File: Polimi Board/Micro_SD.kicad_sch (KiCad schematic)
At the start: 6 parts, among them J3 Micro_SD_Card, U4 74LVC125

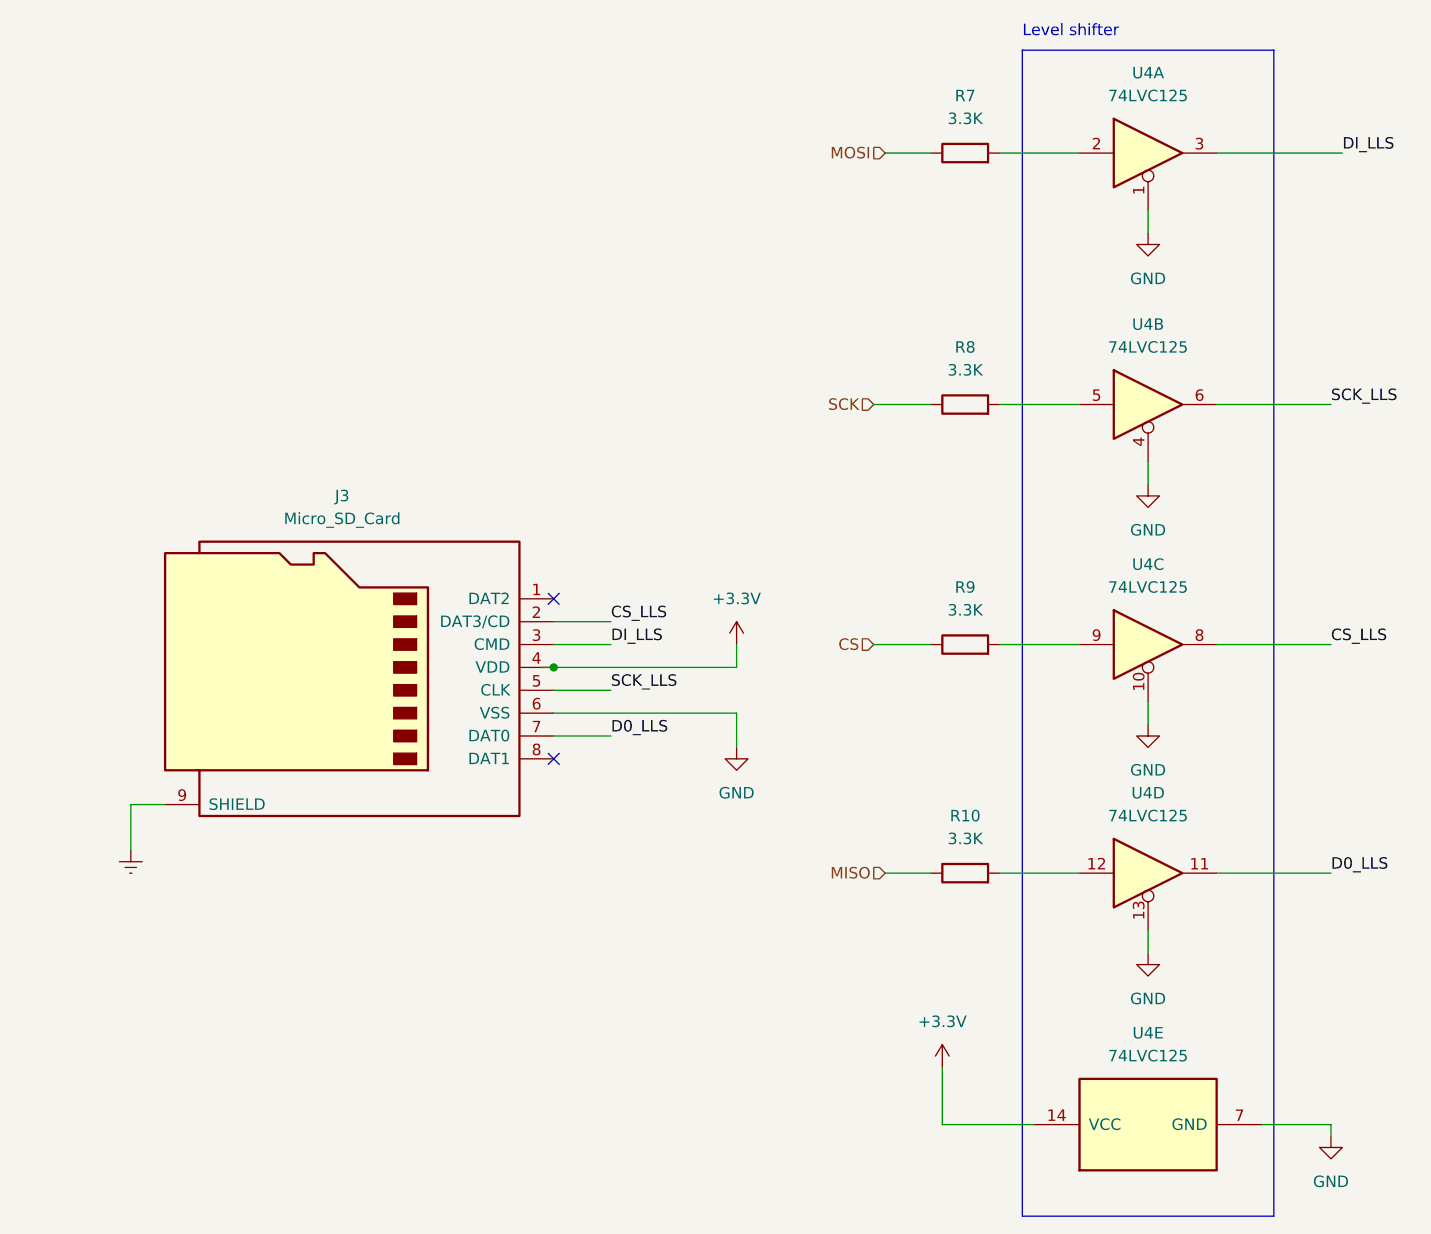
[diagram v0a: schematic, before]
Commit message: Fatte modifiche
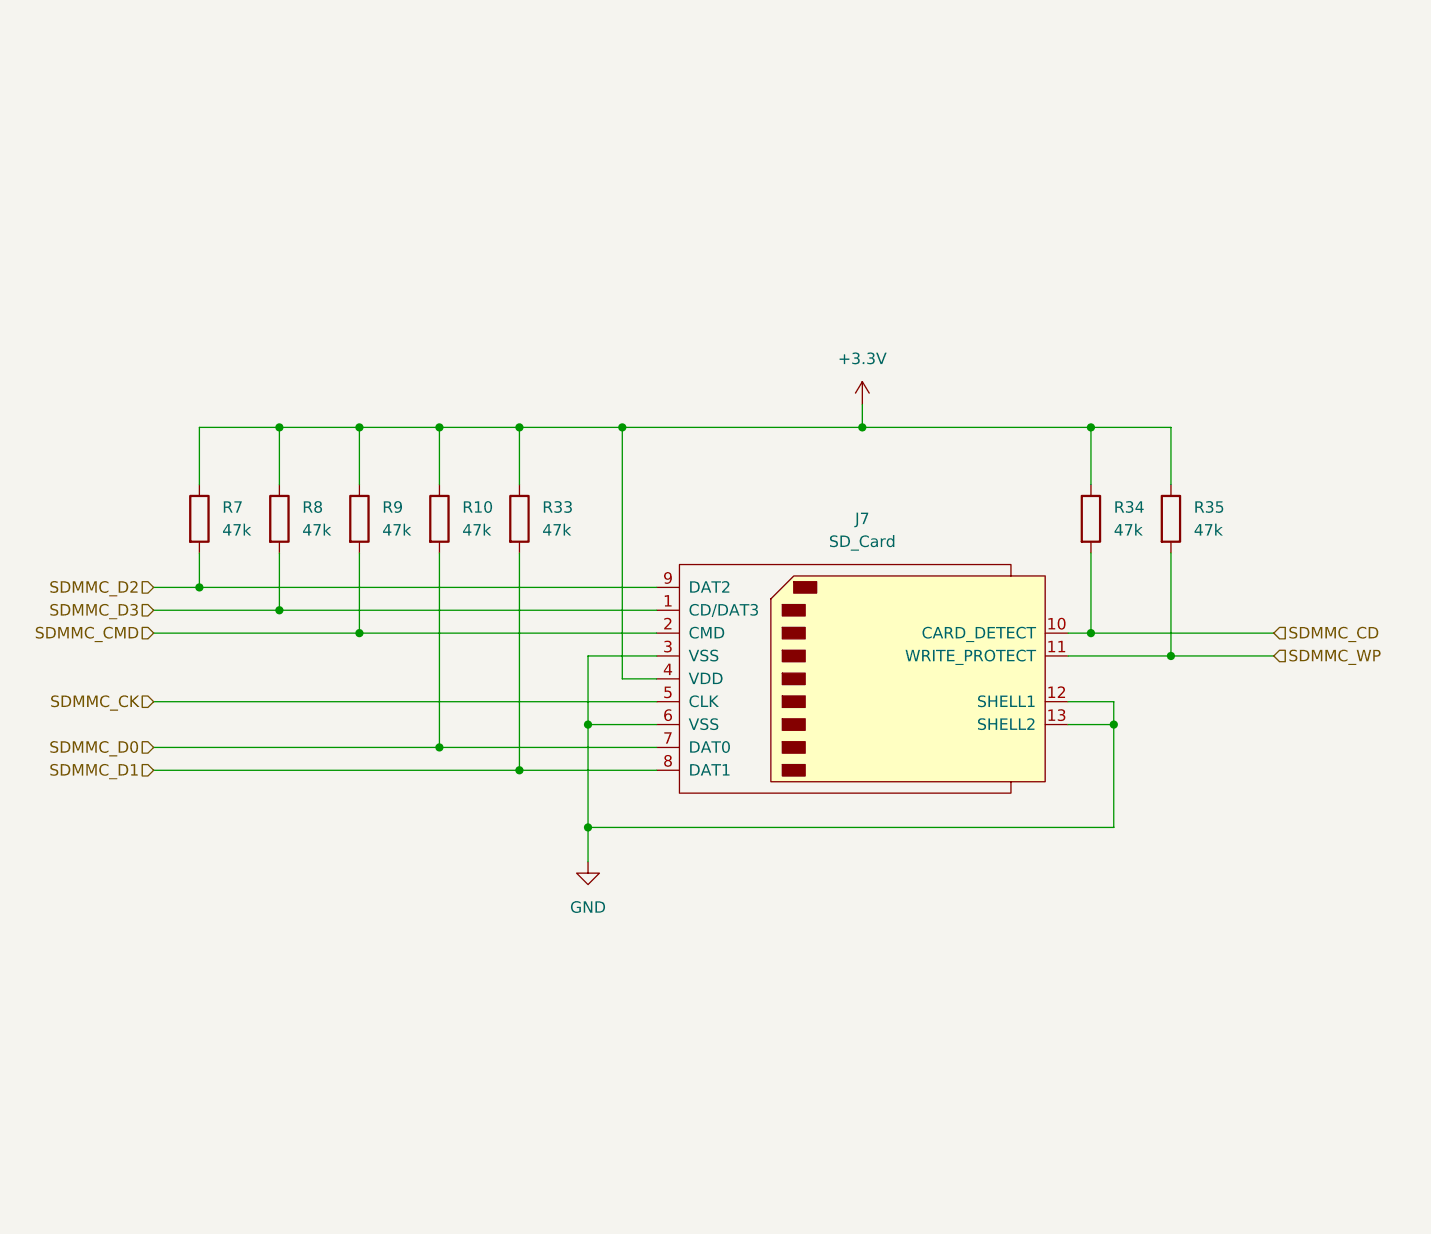
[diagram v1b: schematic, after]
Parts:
- removed J3: Micro_SD_Card, symbol Connector:Micro_SD_Card
- removed U4: 74LVC125, symbol 74xx:74LVC125
- added J7: SD_Card, symbol Connector:SD_Card
- added R33, R34, R35: 47k, symbol Device:R
- R10, R7, R8, R9: value 3.3K -> 47k
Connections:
- net CS is gone; now on net +3.3V: R9.1
- net MISO is gone; now on net +3.3V: R10.1
- net MOSI is gone; now on net +3.3V: R7.1
- net SCK is gone; now on net +3.3V: R8.1
- net +3.3V: now also J7.4 (VDD), R33.1, R34.1, R35.1
- net GND: now also J7.12 (SHELL1), J7.13 (SHELL2), J7.3 (VSS), J7.6 (VSS)
- net SDMMC_D2: now reaches R7.2
- net SDMMC_D2: now also J7.9 (DAT2)
- net SDMMC_D0: now reaches R10.2
- net SDMMC_D0: now also J7.7 (DAT0)
- net SDMMC_D3: now reaches R8.2
- net SDMMC_D3: now also J7.1 (CD/DAT3)
- net SDMMC_CMD: now reaches R9.2
- net SDMMC_CMD: now also J7.2 (CMD)
- new net SDMMC_CD: J7.10 (CARD_DETECT), R34.2
- new net SDMMC_CK: J7.5 (CLK)
- new net SDMMC_D1: J7.8 (DAT1), R33.2
- new net SDMMC_WP: J7.11 (WRITE_PROTECT), R35.2
- no-connect marks 2 -> 0
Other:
- note removed: "Level shifter"
